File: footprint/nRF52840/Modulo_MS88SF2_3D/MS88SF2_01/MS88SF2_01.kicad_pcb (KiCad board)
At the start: 2 copper layers, 17.4 x 23.2 mm, 21 parts, among them U1 MS88SF2-castellate

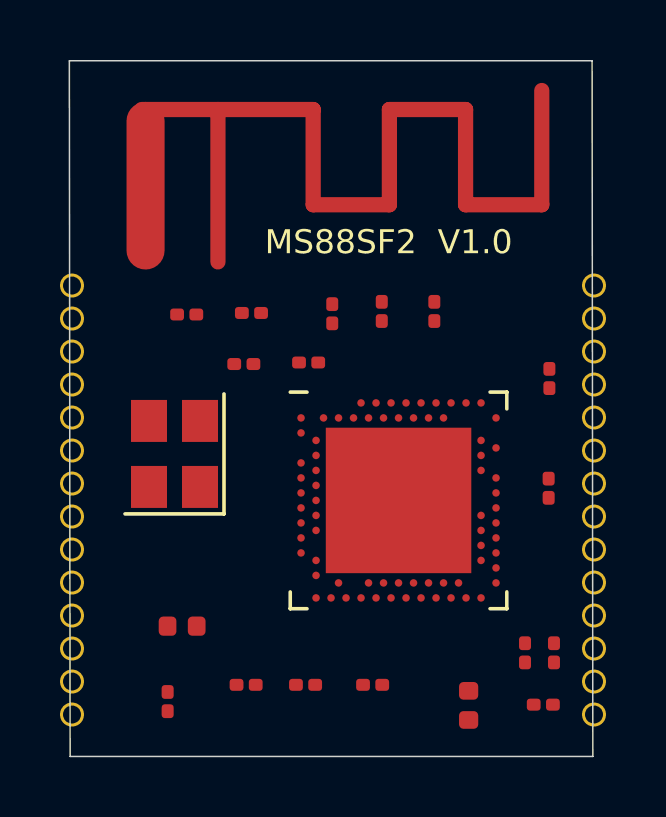
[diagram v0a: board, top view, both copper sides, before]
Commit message: update
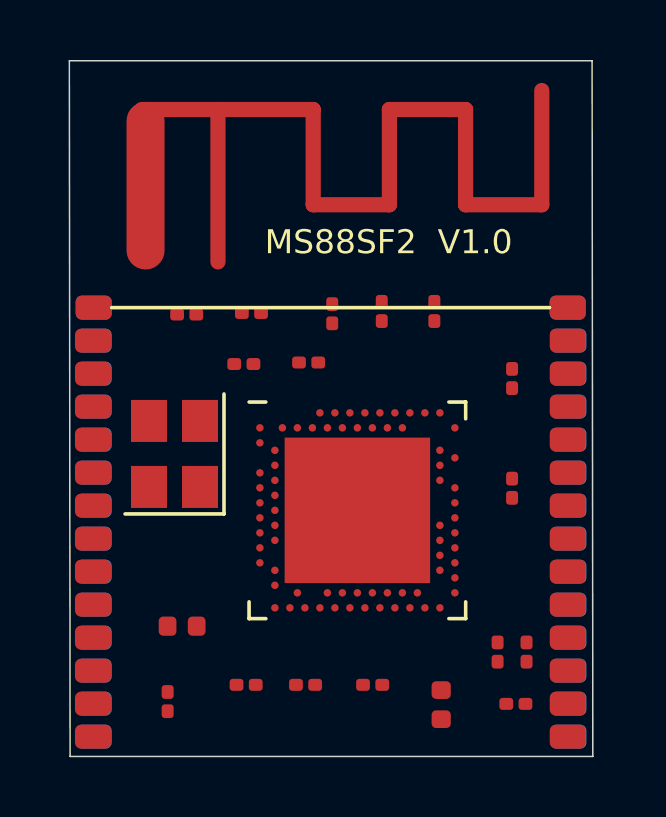
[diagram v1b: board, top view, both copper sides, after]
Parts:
- removed U1: MS88SF2-castellate, MS88SF2_01:MS88SF2-castellate
- added REF**: MS88SF2_v2, MS88SF2_01:MS88SF2_v2, B.Cu at (147.5, 98.7)
- added REF**: MS88SF2_v2, MS88SF2_01:MS88SF2_v2, F.Cu at (131.7, 98.7)
- moved REF** 1.41 mm to (140.5, 105.4)
- moved REF** 1.24 mm to (145.7, 101.0)
- moved REF** 1.22 mm to (145.7, 104.7)
- moved REF** 0.91 mm to (145.8, 111.9)
- moved REF** 0.91 mm to (146.2, 110.2)
- moved REF** 0.91 mm to (145.2, 110.2)
- moved REF** 0.91 mm to (143.3, 111.9)
